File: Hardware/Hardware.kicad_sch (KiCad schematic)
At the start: 1 part, among them U1 Teensy4.1_DEV-16771

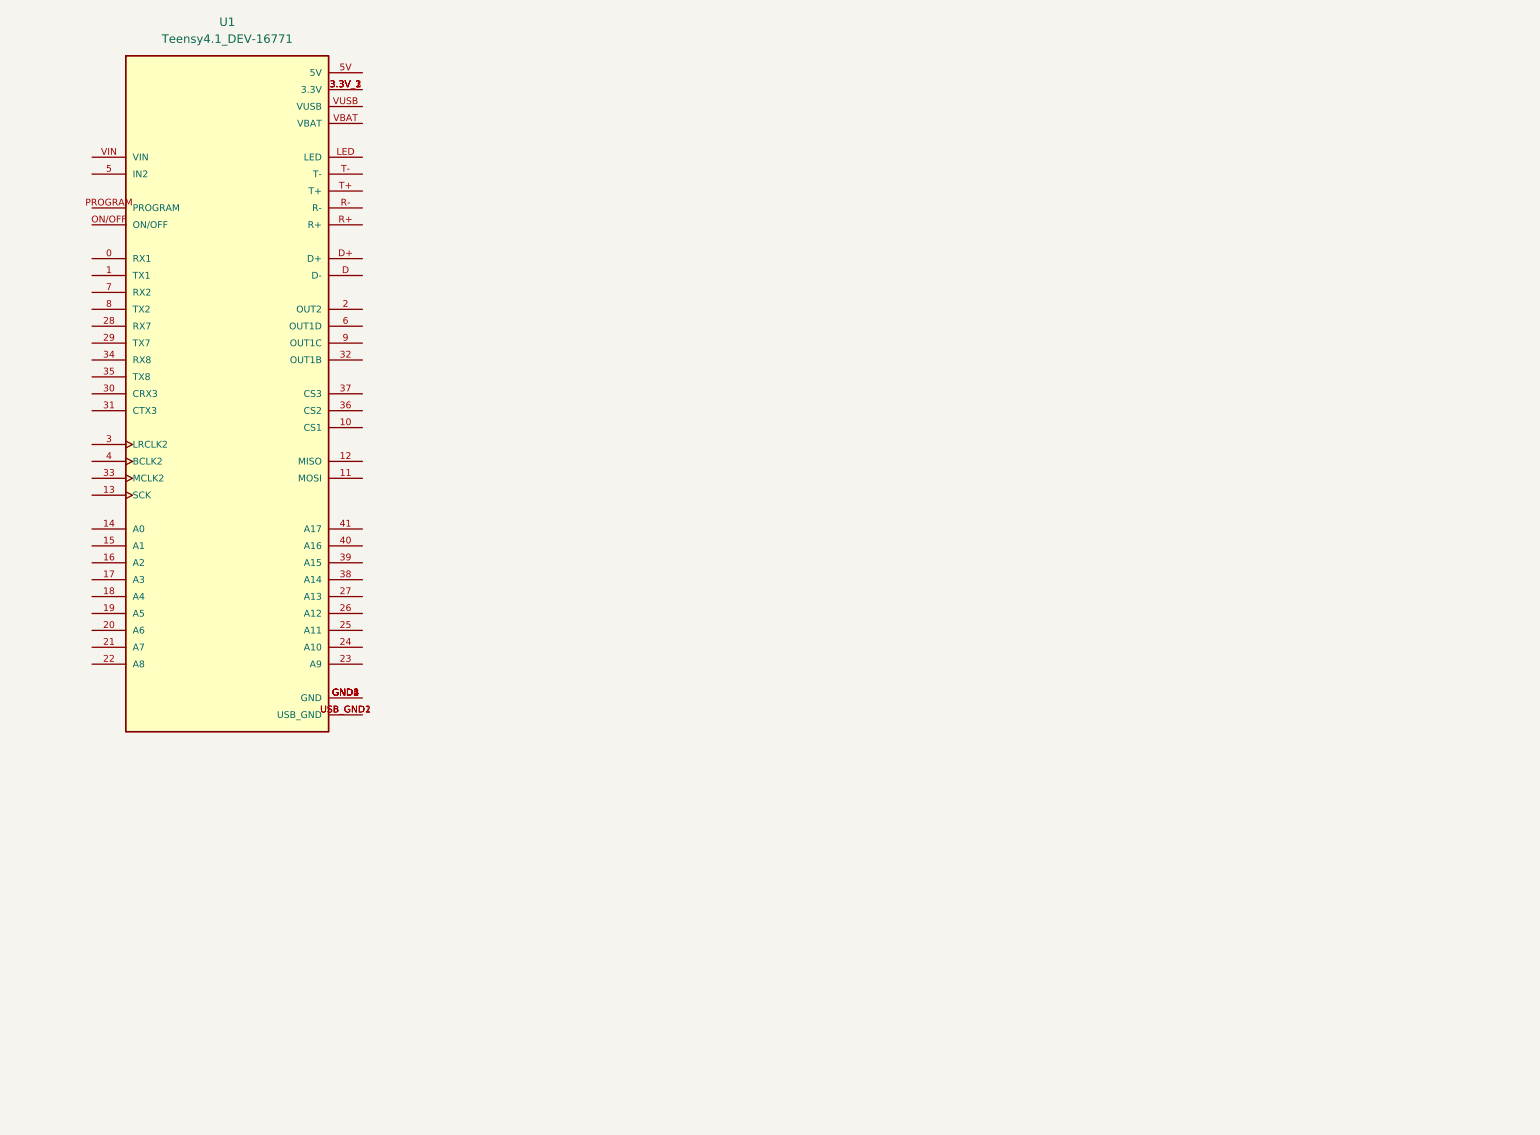
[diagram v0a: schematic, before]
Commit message: Added things (very nice)
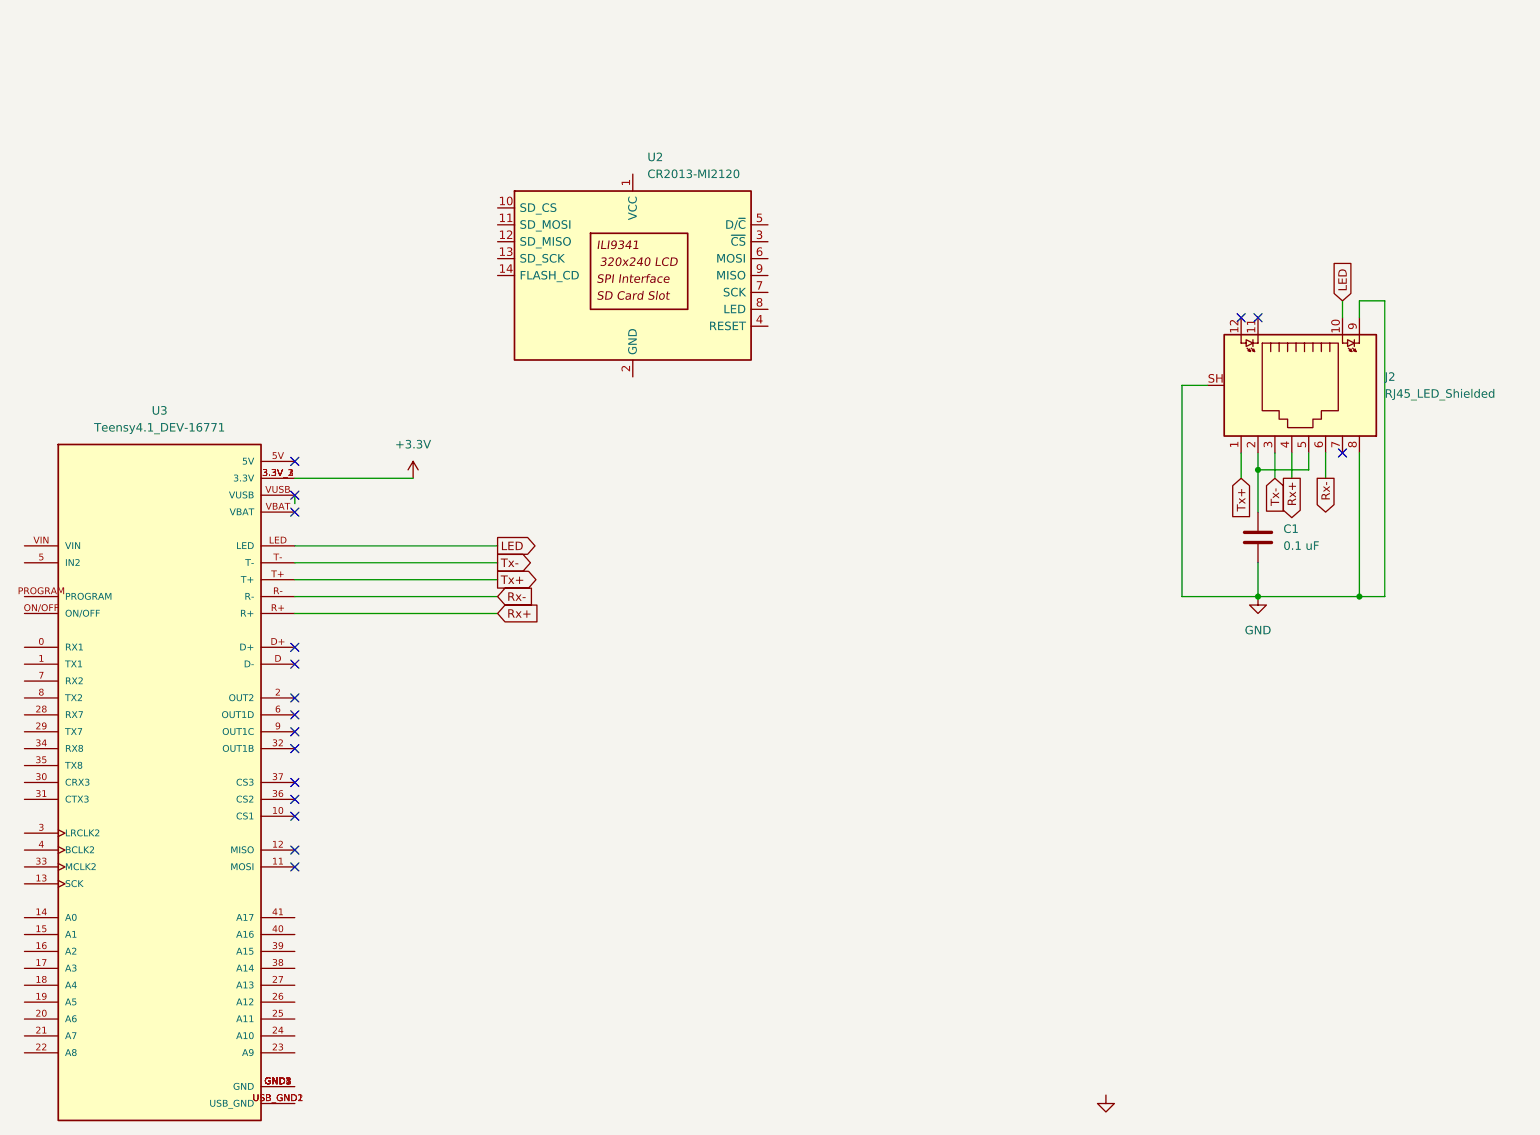
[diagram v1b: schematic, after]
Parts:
- removed U1: Teensy4.1_DEV-16771, MODULE_DEV-16771, symbol MRDT_Shields:Teensy4.1_DEV-16771
- added C1: 0.1 uF, symbol Device:C
- added J2: RJ45_LED_Shielded, symbol Connector:RJ45_LED_Shielded
- added U2: CR2013-MI2120, Display:CR2013-MI2120, symbol Driver_Display:CR2013-MI2120
- added U3: Teensy4.1_DEV-16771, MODULE_DEV-16771, symbol MRDT_Shields:Teensy4.1_DEV-16771
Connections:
- new net: C1.1, J2.2, J2.5
- new net: U3.GND1 (GND), U3.GND2 (GND), U3.GND3 (GND), U3.GND4 (GND), U3.GND5 (GND)
- new net: U3.USB_GND1 (USB_GND), U3.USB_GND2 (USB_GND)
- new net +3.3V: U3.3.3V_1 (3.3V), U3.3.3V_2 (3.3V), U3.3.3V_3 (3.3V)
- new net GND: C1.2, J2.8, J2.9, J2.SH
- new net LED: J2.10, U3.LED
- new net Rx+: J2.4, U3.R+
- new net Rx-: J2.6, U3.R-
- new net Tx+: J2.1, U3.T+
- new net Tx-: J2.3, U3.T-
- no-connect marks 0 -> 17
